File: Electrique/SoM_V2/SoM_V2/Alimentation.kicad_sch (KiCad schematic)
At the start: 1 part

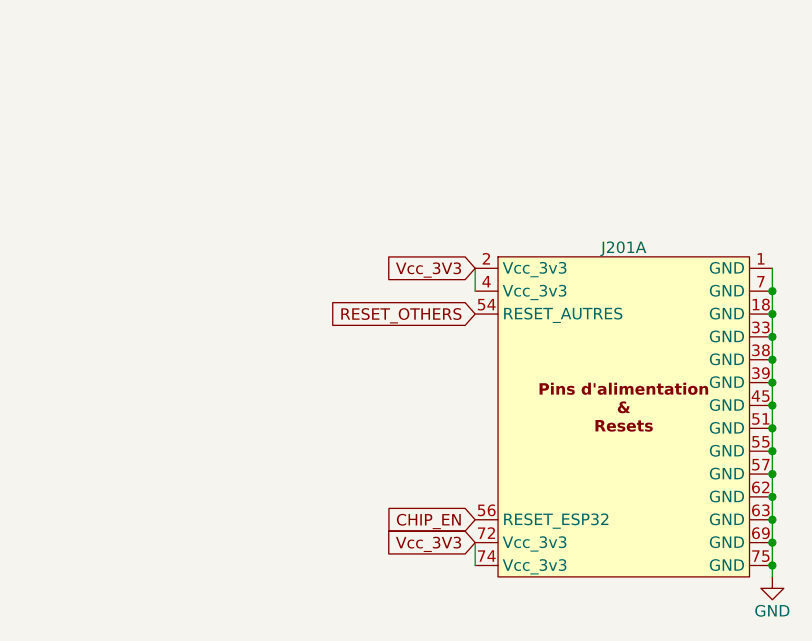
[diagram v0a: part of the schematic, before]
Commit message: push fix ???
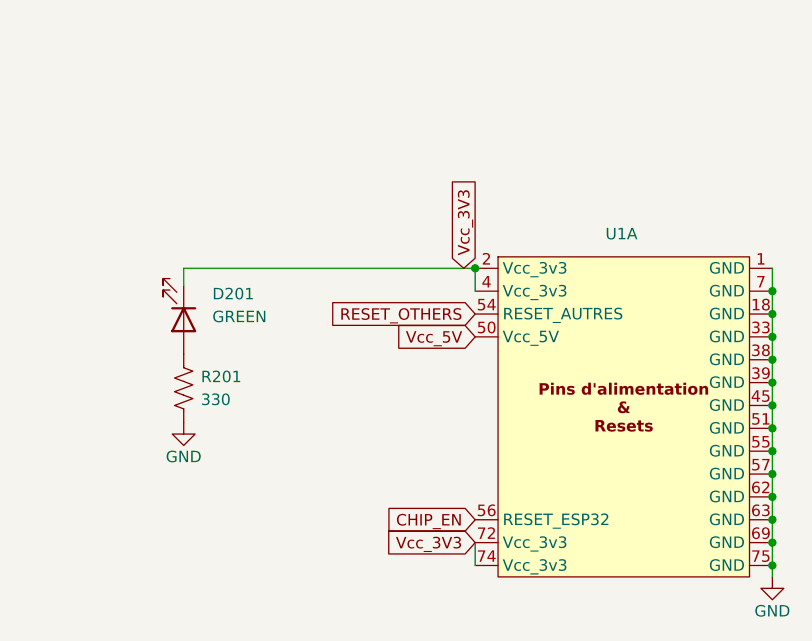
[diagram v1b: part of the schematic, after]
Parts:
- removed J201: ~, connecteur_M2_key_E:NGFF_E, symbol connecteur_m2_key_E:connecteur_SOM_ESP32
- added D201: GREEN, LED_SMD:LED_0805_2012Metric, symbol Device:LED
- added R201: 330, Resistor_SMD:R_0805_2012Metric, symbol Device:R_US
- added U1: ~, connecteur_M2_key_E:NGFF_E, symbol connecteur_m2_key_E:connecteur_SOM_ESP32_V2
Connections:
- net +3V3: now also D201.1 (K), U1.2 (Vcc_3v3), U1.4 (Vcc_3v3), U1.72 (Vcc_3v3), U1.74 (Vcc_3v3)
- net CHIP_EN: now also U1.56 (RESET_ESP32)
- net GND: now also R201.2, U1.1 (GND), U1.18 (GND), U1.33 (GND), U1.38 (GND), U1.39 (GND), U1.45 (GND), U1.51 (GND), U1.55 (GND), U1.57 (GND), U1.62 (GND), U1.63 (GND), U1.69 (GND), U1.7 (GND), U1.75 (GND)
- net RESET_OTHERS: now also U1.54 (RESET_AUTRES)
- new net: D201.2 (A), R201.1
- new net Vcc_5V: U1.50 (Vcc_5V)
